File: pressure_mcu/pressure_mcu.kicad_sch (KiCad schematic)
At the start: 23 parts, among them J1 USB_C_Receptacle_USB2.0_14P, J4 Connector 1, J5 Connector 2, J6 Connector 3, J7 Connector 4, U1 STM32H563RITx, U2 AP2112K-3.3

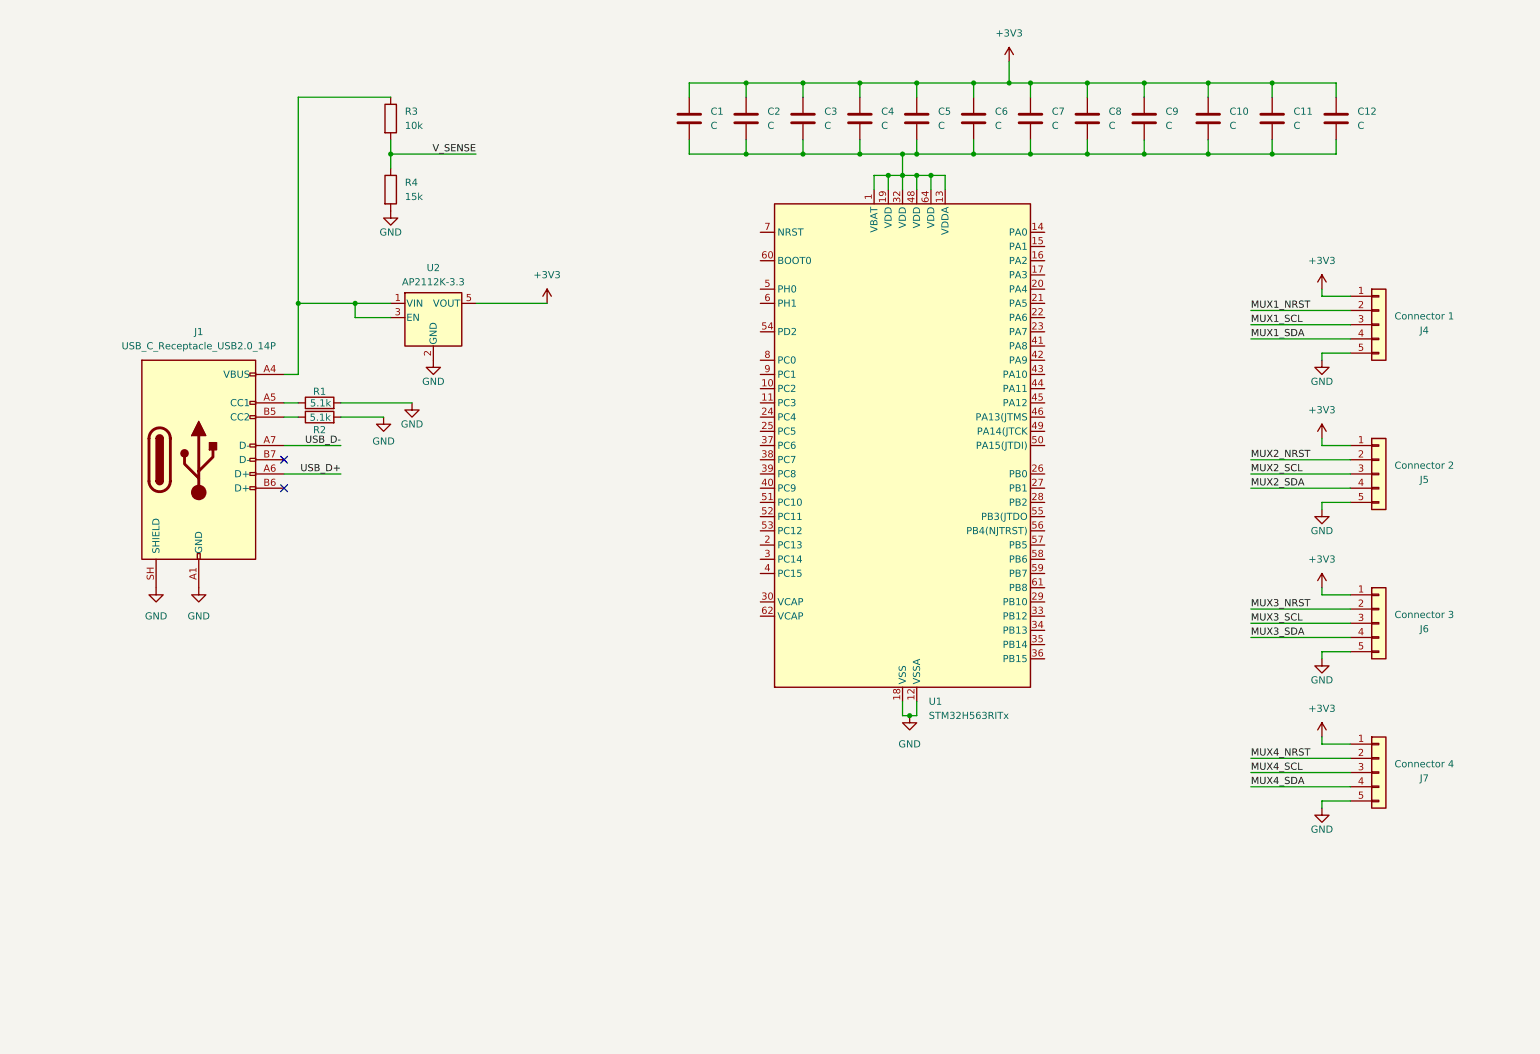
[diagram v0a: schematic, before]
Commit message: strips done, finishing off mcu
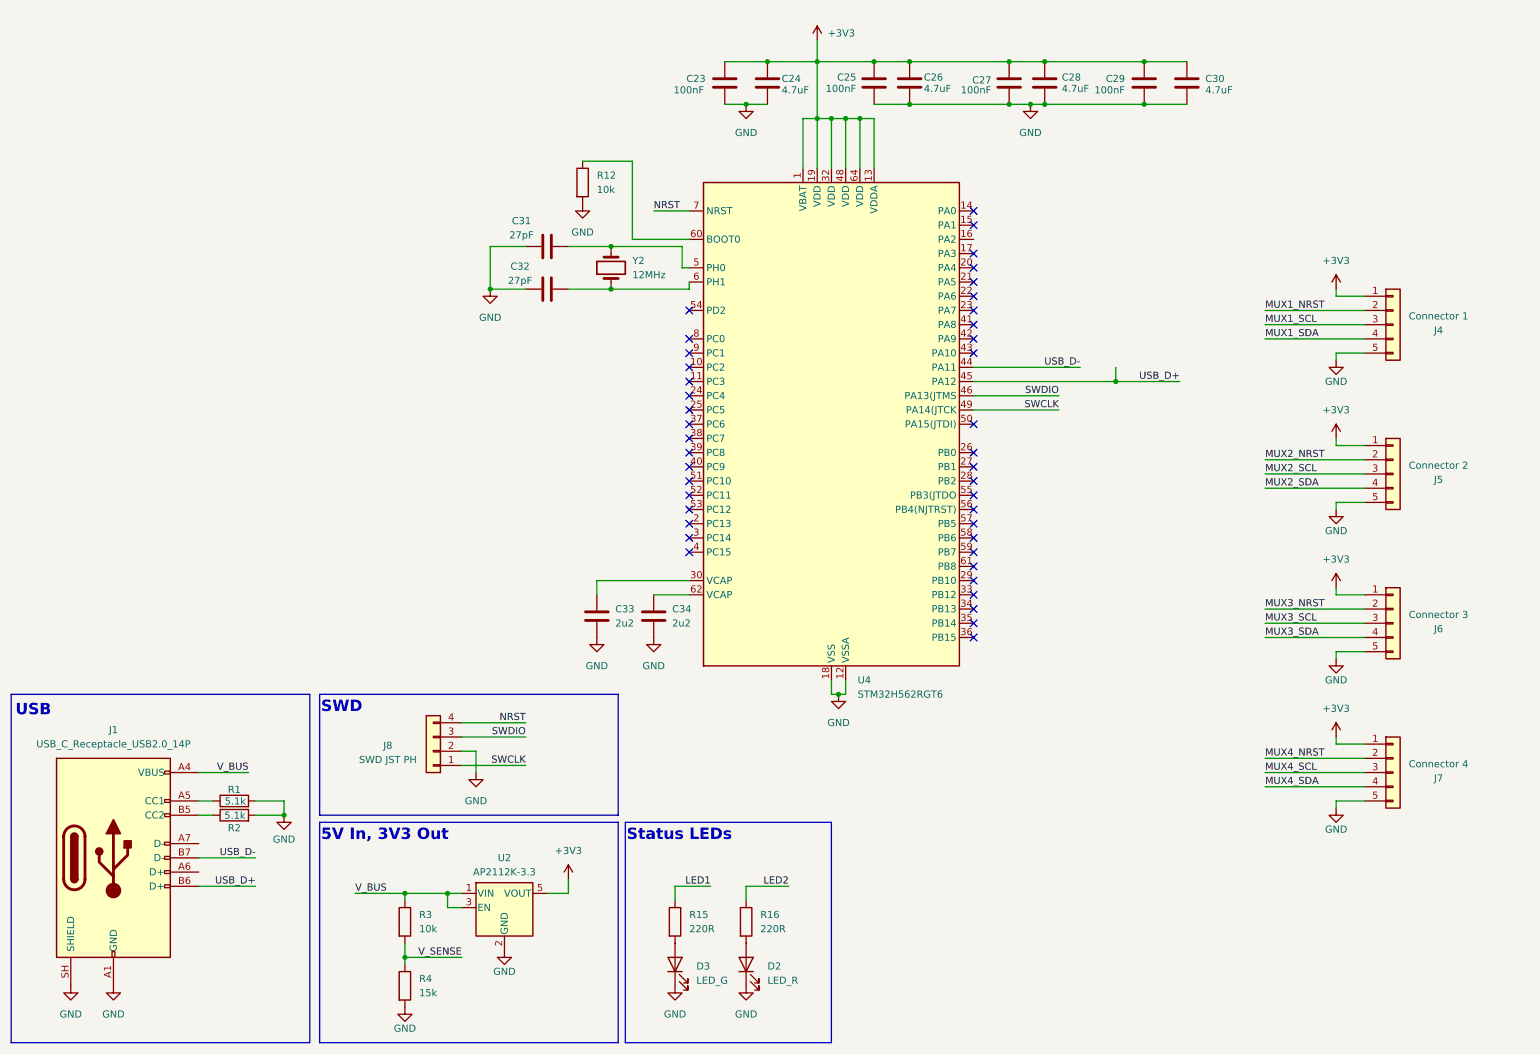
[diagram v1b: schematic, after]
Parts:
- removed C1, C10, C11, C12, C2, C3, C4, C5, C6, C7, C8, C9: C, Capacitor_SMD:C_0402_1005Metric, symbol Device:C
- removed U1: STM32H563RITx, Package_QFP:LQFP-64_10x10mm_P0.5mm, symbol MCU_ST_STM32H5:STM32H563RITx
- added C23, C25, C27, C29: 100nF, Capacitor_SMD:C_0603_1608Metric, symbol Device:C
- added C24, C26, C28, C30: 4.7uF, Capacitor_SMD:C_0603_1608Metric, symbol Device:C
- added C31, C32: 27pF, Capacitor_SMD:C_0603_1608Metric, symbol Device:C
- added C33, C34: 2u2, Resistor_SMD:R_0603_1608Metric, symbol Device:C
- added D2: LED_R, LED_SMD:LED_0603_1608Metric, symbol Device:LED
- added D3: LED_G, LED_SMD:LED_0603_1608Metric, symbol Device:LED
- added J8: SWD JST PH, Connector_JST:JST_PH_B4B-PH-K_1x04_P2.00mm_Vertical, symbol Connector_Generic:Conn_01x04
- added R12: 10k, Resistor_SMD:R_0603_1608Metric, symbol Device:R
- added R15, R16: 220R, Resistor_SMD:R_0603_1608Metric, symbol Device:R
- added U4: STM32H562RGT6, Package_QFP:LQFP-64_10x10mm_P0.5mm, symbol MCU_ST_STM32H5:STM32H562RGTx
- added Y2: 12MHz, Crystal:Crystal_SMD_Abracon_ABM8G-4Pin_3.2x2.5mm, symbol Device:Crystal
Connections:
- net +3V3: now also C23.1, C24.1, C25.1, C26.1, C27.1, C28.1, C29.1, C30.1, U4.1 (VBAT), U4.13 (VDDA), U4.19 (VDD), U4.32 (VDD), U4.48 (VDD), U4.64 (VDD)
- net GND: now also C23.2, C24.2, C25.2, C26.2, C27.2, C28.2, C29.2, C30.2, C31.1, C32.2, C33.2, C34.2, D2.1 (K), D3.1 (K), J8.2 (Pin_2), R12.2, U4.12 (VSSA), U4.18 (VSS), U4.31 (VSS), U4.47 (VSS), U4.63 (VSS)
- net USB_D+: now also J1.B6 (D+), U4.45 (PA12); no longer J1.A6 (D+)
- net USB_D-: now also J1.B7 (D-), U4.44 (PA11); no longer J1.A7 (D-)
- net V_BUS: now reaches J1.A4 (VBUS), J1.A9 (VBUS), J1.B4 (VBUS), J1.B9 (VBUS), R3.1, U2.1 (VIN), U2.3 (EN)
- new net: R12.1, U4.60 (BOOT0)
- new net: C33.1, U4.30 (VCAP)
- new net: D3.2 (A), R15.2
- new net: C31.2, U4.5 (PH0), Y2.3 (2)
- new net: C32.1, U4.6 (PH1), Y2.1
- new net: C34.1, U4.62 (VCAP)
- new net: D2.2 (A), R16.2
- new net LED1: R15.1
- new net LED2: R16.1
- new net NRST: J8.4 (Pin_4), U4.7 (NRST)
- new net SWCLK: J8.1 (Pin_1), U4.49 (PA14(JTCK)
- new net SWDIO: J8.3 (Pin_3), U4.46 (PA13(JTMS)
- no-connect marks 2 -> 42
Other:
- note added: "5V In, 3V3 Out"
- note added: "SWD"
- note added: "Status LEDs"
- note added: "USB"
- moved on the sheet: J1, J4, J5, J6, J7, R1, R2, U2

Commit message: pressure mcu schematic almost done
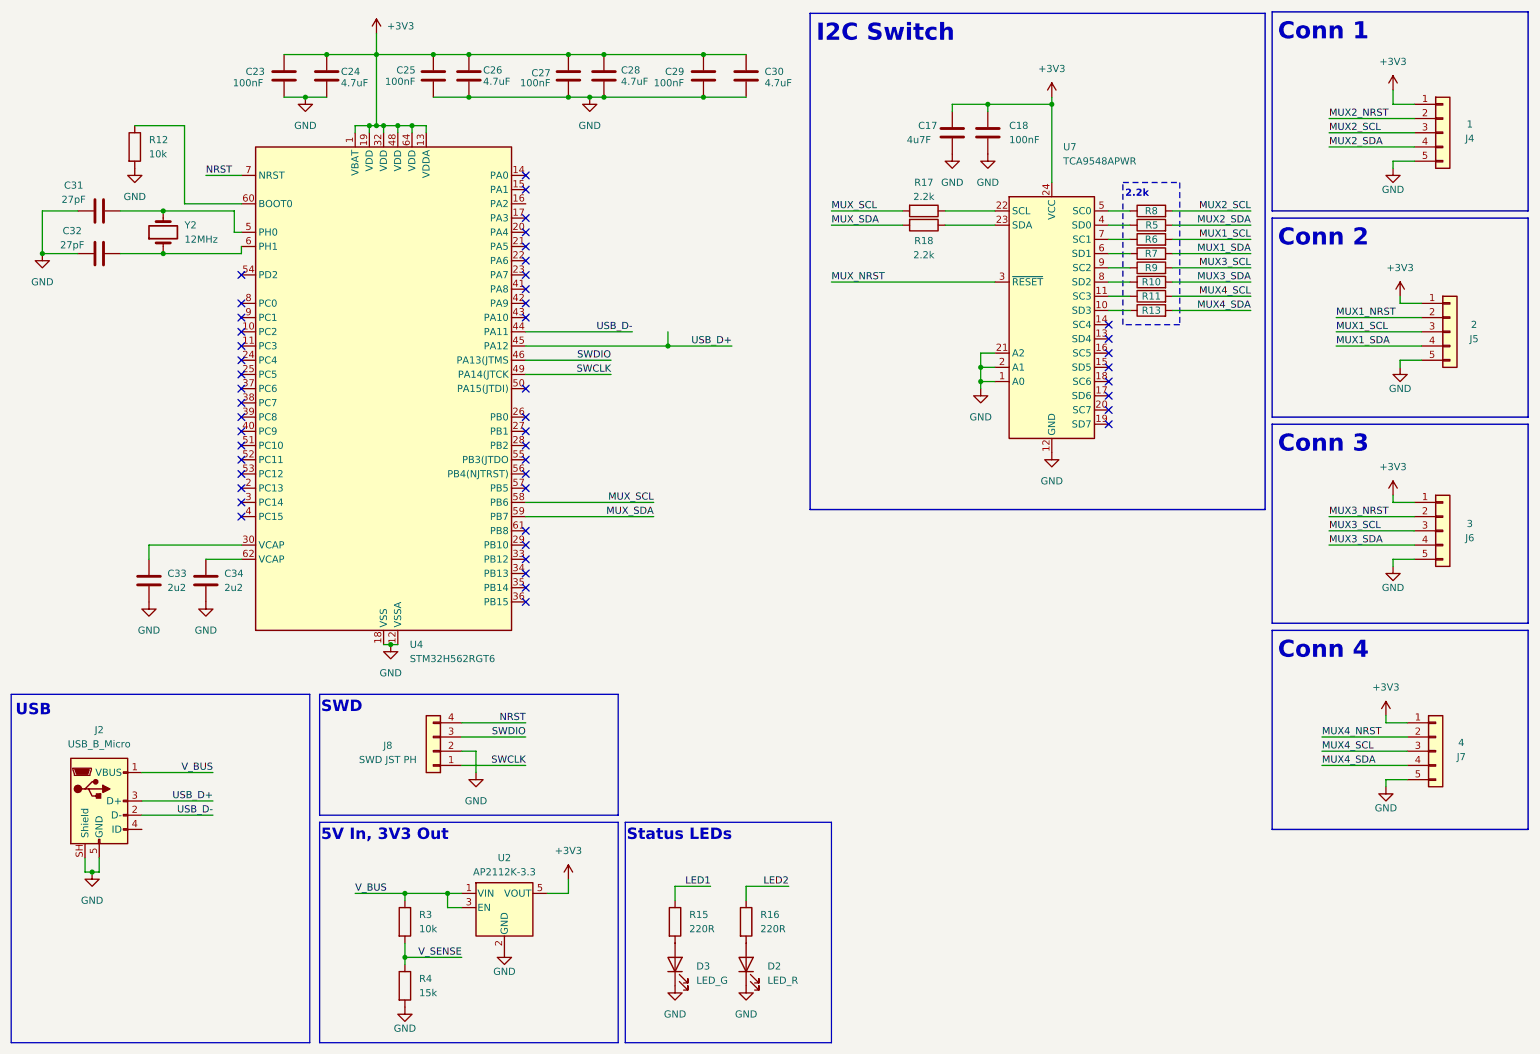
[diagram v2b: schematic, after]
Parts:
- removed J1: USB_C_Receptacle_USB2.0_14P, Connector_USB:USB_C_Receptacle_Amphenol_124019772112A, symbol Connector:USB_C_Receptacle_USB2.0_14P
- removed R1, R2: 5.1k, Resistor_SMD:R_0402_1005Metric, symbol Device:R
- added C17: 4u7F, Capacitor_SMD:C_0402_1005Metric, symbol Device:C
- added C18: 100nF, Capacitor_SMD:C_0402_1005Metric, symbol Device:C
- added J2: USB_B_Micro, Connector_USB:USB_Micro-B_Amphenol_10118193-0001LF_Horizontal, symbol Connector:USB_B_Micro
- added R10, R11, R13, R5, R6, R7, R8, R9: R, Resistor_SMD:R_0402_1005Metric, symbol Device:R
- added R17, R18: 2.2k, Resistor_SMD:R_0402_1005Metric, symbol Device:R
- added U7: TCA9548APWR, Package_SO:TSSOP-24_4.4x7.8mm_P0.65mm, symbol Interface_Expansion:TCA9548APWR
- J4: value Connector 1 -> 1; footprint Connector_JST:JST_EH_B5B-EH-A_1x05_P2.50mm_Vertical -> Connector_Wuerth:Wuerth_WR-WTB_64800511622_1x05_P1.50mm_Vertical
- J5: value Connector 2 -> 2; footprint Connector_JST:JST_EH_B5B-EH-A_1x05_P2.50mm_Vertical -> Connector_Wuerth:Wuerth_WR-WTB_64800511622_1x05_P1.50mm_Vertical
- J6: value Connector 3 -> 3; footprint Connector_JST:JST_EH_B5B-EH-A_1x05_P2.50mm_Vertical -> Connector_Wuerth:Wuerth_WR-WTB_64800511622_1x05_P1.50mm_Vertical
- J7: value Connector 4 -> 4; footprint Connector_JST:JST_EH_B5B-EH-A_1x05_P2.50mm_Vertical -> Connector_Wuerth:Wuerth_WR-WTB_64800511622_1x05_P1.50mm_Vertical
- J8: footprint Connector_JST:JST_PH_B4B-PH-K_1x04_P2.00mm_Vertical -> Connector:Tag-Connect_TC2050-IDC-NL_2x05_P1.27mm_Vertical_with_bottom_clip
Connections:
- net +3V3: now also C17.1, C18.1, U7.24 (VCC)
- net GND: now also C17.2, C18.2, J2.5 (GND), J2.SH (Shield), U7.1 (A0), U7.12 (GND), U7.2 (A1), U7.21 (A2)
- net MUX1_NRST: now also J5.2 (Pin_2); no longer J4.2 (Pin_2)
- net MUX1_SCL: now also J5.3 (Pin_3), R6.2; no longer J4.3 (Pin_3)
- net MUX1_SDA: now also J5.4 (Pin_4), R7.2; no longer J4.4 (Pin_4)
- net MUX2_NRST: now also J4.2 (Pin_2); no longer J5.2 (Pin_2)
- net MUX2_SCL: now also J4.3 (Pin_3), R8.2; no longer J5.3 (Pin_3)
- net MUX2_SDA: now also J4.4 (Pin_4), R5.2; no longer J5.4 (Pin_4)
- net MUX3_SCL: now also R9.2
- net MUX3_SDA: now also R10.2
- net MUX4_SCL: now also R11.2
- net MUX4_SDA: now also R13.2
- net USB_D+: now also J2.3 (D+)
- net USB_D-: now also J2.2 (D-)
- net V_BUS: now also J2.1 (VBUS)
- net MUX_SCL: now reaches U4.58 (PB6)
- net MUX_SCL: now also R17.2
- net MUX_SDA: now reaches U4.59 (PB7)
- net MUX_SDA: now also R18.2
- new net: R6.1, U7.7 (SC1)
- new net: R7.1, U7.6 (SD1)
- new net: R18.1, U7.23 (SDA)
- new net: R17.1, U7.22 (SCL)
- new net: R10.1, U7.8 (SD2)
- new net: R13.1, U7.10 (SD3)
- new net: R11.1, U7.11 (SC3)
- new net: R5.1, U7.4 (SD0)
- new net: R8.1, U7.5 (SC0)
- new net: R9.1, U7.9 (SC2)
- new net MUX_NRST: U7.3 (~{RESET})
- no-connect marks 42 -> 48
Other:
- note added: "2.2k"
- note added: "Conn 1"
- note added: "Conn 2"
- note added: "Conn 3"
- note added: "Conn 4"
- note added: "I2C Switch"
- moved on the sheet: C23, C24, C25, C26, C27, C28, C29, C30, C31, C32, C33, C34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
